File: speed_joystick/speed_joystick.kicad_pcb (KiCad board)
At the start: 2 copper layers, 89.2 x 61.1 mm, 67 parts, among them SW1 JS5208, U1 Teensy3.2, U2 SN65HVD230

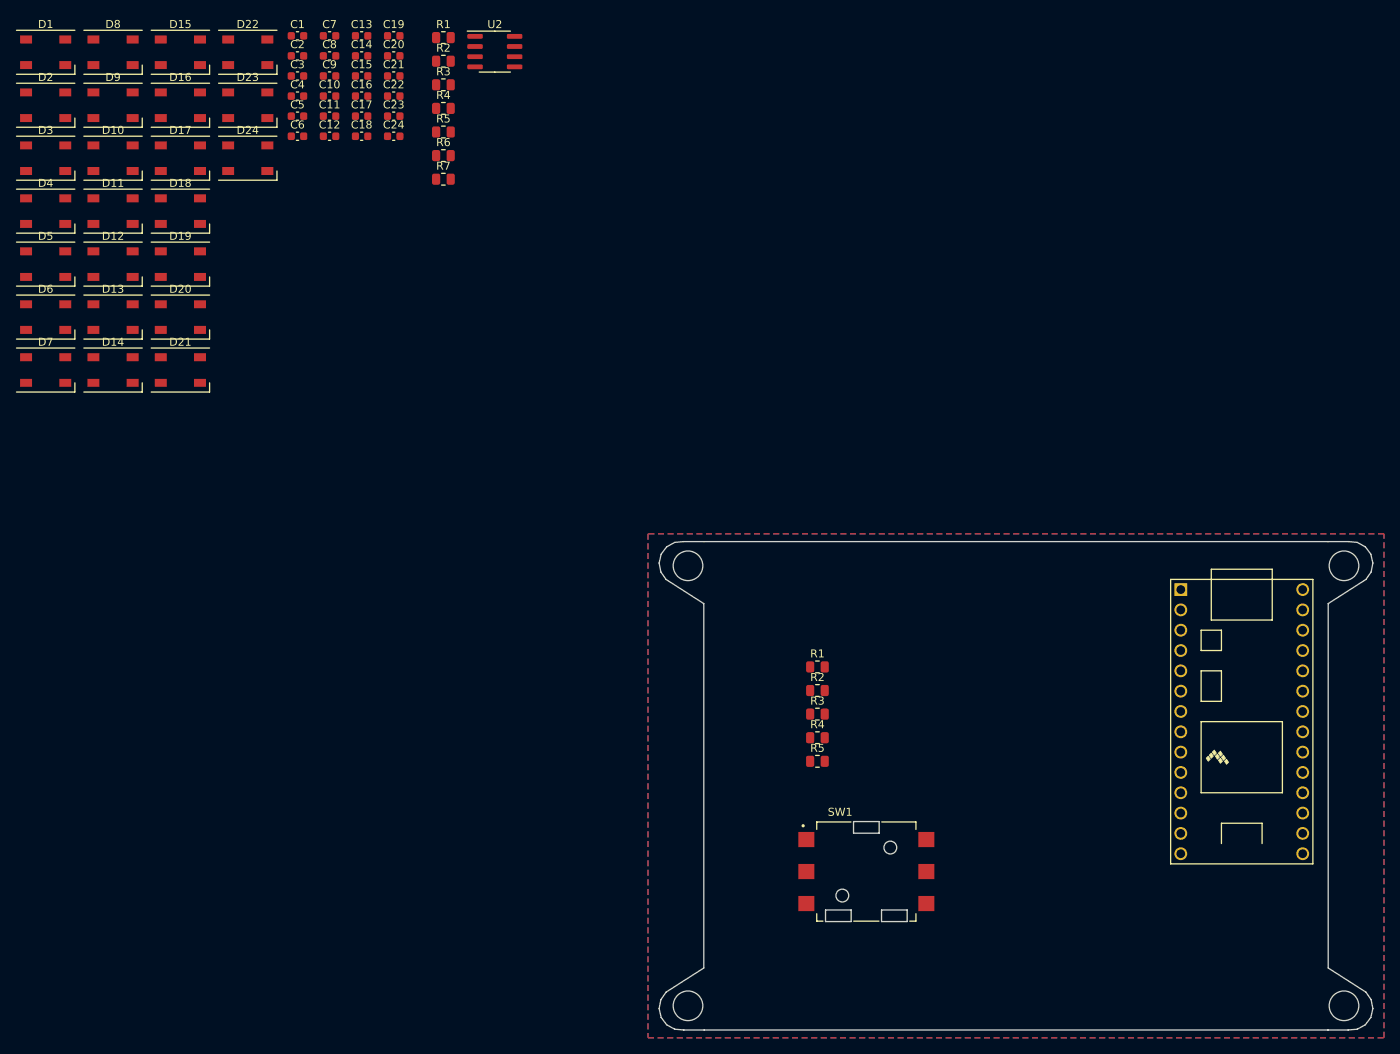
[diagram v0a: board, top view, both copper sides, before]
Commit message: work on speed_joystick pcb
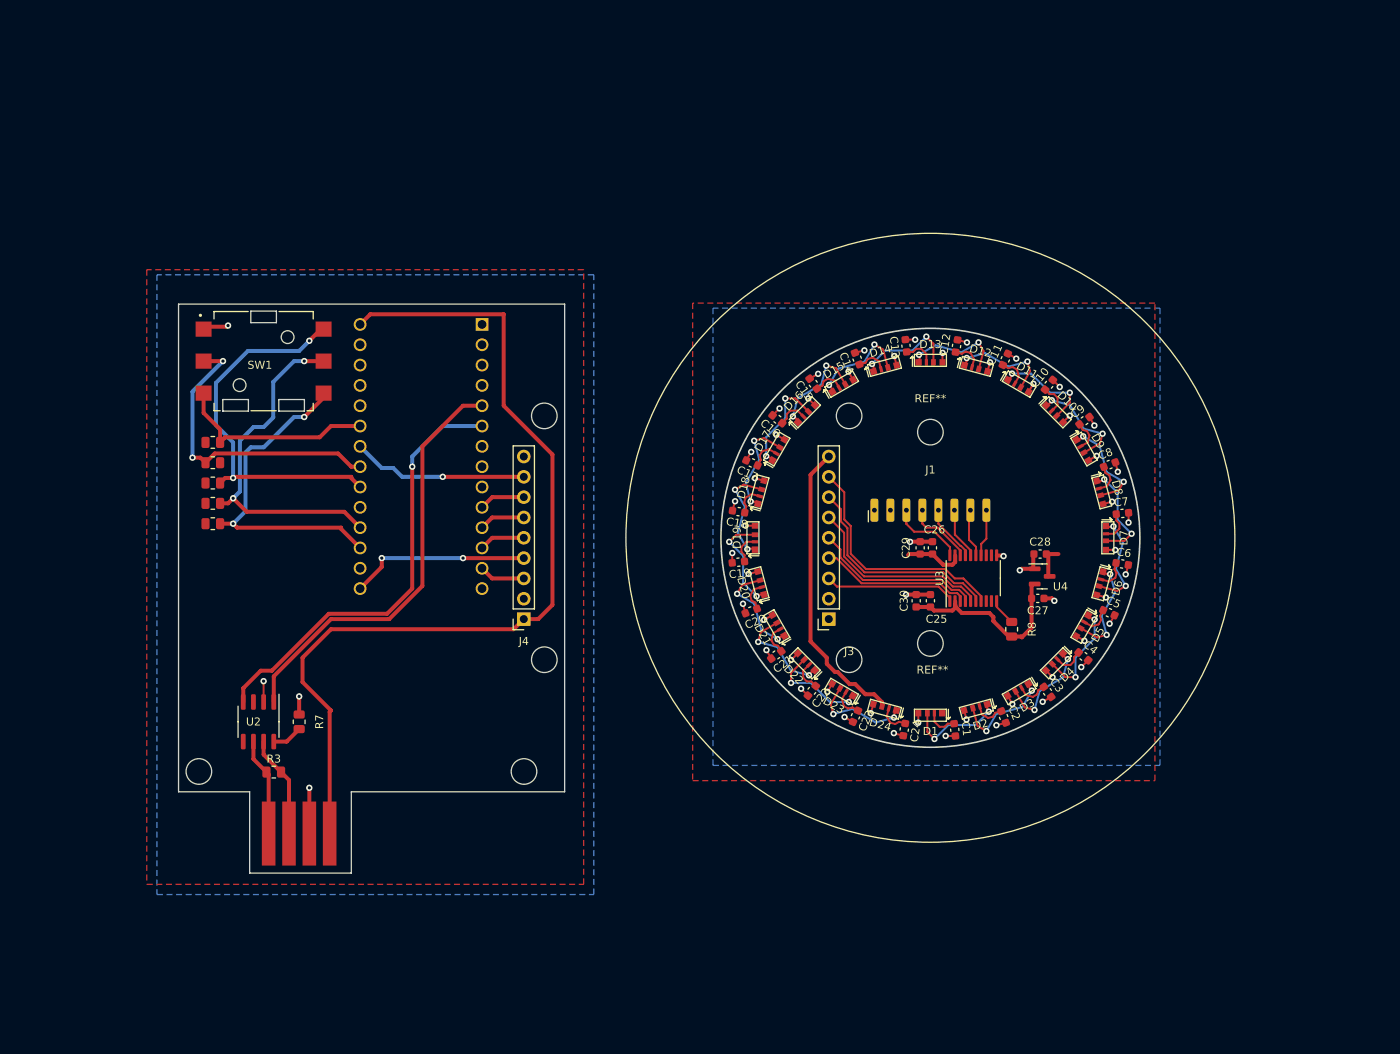
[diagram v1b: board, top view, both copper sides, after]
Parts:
- removed the R1 at (53.4, 0.97)
- removed the R1 at (100.2, 79.6)
- removed the R2 at (53.4, 3.92)
- removed the R2 at (100.2, 82.6)
- removed the R3 at (100.2, 85.5)
- removed the R3 at (53.4, 6.88)
- removed the R4 at (53.4, 9.82)
- removed the R4 at (100.2, 88.5)
- removed the R5 at (100.2, 91.4)
- removed the R5 at (53.4, 12.8)
- removed the REF** at (84.0, 67.0)
- removed the REF** at (84.0, 122.0)
- removed the REF** at (166.0, 122.0)
- removed the REF** at (166.0, 67.0)
- added ?: , , F.Cu at (66.0, 48.3)
- added ?: , , F.Cu at (63.5, 92.7)
- added ?: , , F.Cu at (104.1, 78.7)
- added ?: , , F.Cu at (66.0, 78.7)
- added ?: , , F.Cu at (104.1, 48.3)
- added ?: , , F.Cu at (22.9, 92.7)
- added C25: 0.1uF, Capacitor_SMD:C_0603_1608Metric, F.Cu at (114.3, 71.4)
- added C26: 0.1uF, Capacitor_SMD:C_0603_1608Metric, F.Cu at (114.6, 64.8)
- added C27: 1uF, Capacitor_SMD:C_0603_1608Metric, F.Cu at (127.7, 71.1)
- added C28: 1uF, Capacitor_SMD:C_0603_1608Metric, F.Cu at (128.0, 65.5)
- added C29: 10uF, Capacitor_SMD:C_0603_1608Metric, F.Cu at (113.0, 64.8)
- added C30: 10uF, Capacitor_SMD:C_0603_1608Metric, F.Cu at (112.5, 71.4)
- added J1: Conn_01x08, 8_hole:8_hole, F.Cu at (114.3, 60.0)
- added J2: Conn_01x04, 4pin:my_4_tab_edge, F.Cu at (31.6, 100.5)
- added J3: Conn_01x09, Connector_PinSocket_2.54mm:PinSocket_1x09_P2.54mm_Vertical, F.Cu at (101.6, 73.7)
- added J4: Conn_01x09, Connector_PinSocket_2.54mm:PinSocket_1x09_P2.54mm_Vertical, F.Cu at (63.5, 73.7)
- added R1: 10k, Resistor_SMD:R_0805_2012Metric, F.Cu at (24.6, 61.7)
- added R2: 10k, Resistor_SMD:R_0805_2012Metric, F.Cu at (24.6, 59.2)
- added R3: 120, Resistor_SMD:R_0805_2012Metric, F.Cu at (32.2, 92.8)
- added R4: 10k, Resistor_SMD:R_0805_2012Metric, F.Cu at (24.6, 56.7)
- added R5: 10k, Resistor_SMD:R_0805_2012Metric, F.Cu at (24.6, 51.6)
- added R8: R, Resistor_SMD:R_0805_2012Metric, F.Cu at (124.5, 74.9)
- added REF**: MountingHole_3.2mm_M3, MountingHole:MountingHole_3.2mm_M3, F.Cu at (114.3, 50.3)
- added REF**: MountingHole_3.2mm_M3, MountingHole:MountingHole_3.2mm_M3, F.Cu at (114.3, 76.7)
- added U3: 100k, Package_SO:TSSOP-20_4.4x6.5mm_P0.65mm, F.Cu at (119.7, 68.5)
- added U4: XC6206PxxxMR, Package_TO_SOT_SMD:SOT-23, F.Cu at (128.3, 68.3)
- D1, D10, D11, D12, D13, D14, D15, D16, D17, D18, D19, D2, D20, D21, D22, D23, D24, D3, D4, D5, D6, D7, D8, D9: footprint LED_SMD:LED_SK6812_PLCC4_5.0x5.0mm_P3.2mm -> LED_SMD:my_SK6812
- U1: moved to B.Cu
- moved D3 138.7 mm to (125.4, 82.7), turned to -150 degrees
- moved D2 138.7 mm to (120.0, 84.9), turned to -165 degrees
- moved D4 138.3 mm to (130.0, 79.2), turned to -135 degrees
- moved D1 138.2 mm to (114.3, 85.7), turned to 180 degrees
- moved D5 137.5 mm to (133.5, 74.6), turned to -120 degrees
- moved D6 136.2 mm to (135.7, 69.2), turned to -105 degrees
- moved D8 135.3 mm to (135.7, 57.8), turned to -75 degrees
- moved D7 134.4 mm to (136.5, 63.5), turned to -90 degrees
- moved D9 128.8 mm to (133.5, 52.4), turned to -60 degrees
- moved D10 122.1 mm to (130.0, 47.8), turned to -45 degrees
- moved C3 121.3 mm to (128.9, 82.8), turned to -54 degrees
- moved C2 120.9 mm to (123.5, 85.9), turned to -69 degrees
- moved C4 120.6 mm to (133.4, 78.3), turned to -39 degrees
- moved C1 119.5 mm to (117.3, 87.5), turned to -84 degrees
- moved C5 118.9 mm to (136.6, 72.9), turned to -24 degrees
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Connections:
- C1 pad 1: +3.3v -> R_+5V
- C1 pad 2: GND -> R_GND
- C10 pad 1: +3.3v -> R_+5V
- C10 pad 2: GND -> R_GND
- C11 pad 1: +3.3v -> R_+5V
- C11 pad 2: GND -> R_GND
- C12 pad 1: +3.3v -> R_+5V
- C12 pad 2: GND -> R_GND
- C13 pad 1: +3.3v -> R_+5V
- C13 pad 2: GND -> R_GND
- C14 pad 1: +3.3v -> R_+5V
- C14 pad 2: GND -> R_GND
- C15 pad 1: +3.3v -> R_+5V
- C15 pad 2: GND -> R_GND
- C16 pad 1: +3.3v -> R_+5V
- C16 pad 2: GND -> R_GND
- C17 pad 1: +3.3v -> R_+5V
- C17 pad 2: GND -> R_GND
- C18 pad 1: +3.3v -> R_+5V
- C18 pad 2: GND -> R_GND
- C19 pad 1: +3.3v -> R_+5V
- C19 pad 2: GND -> R_GND
- C2 pad 1: +3.3v -> R_+5V
- C2 pad 2: GND -> R_GND
- C20 pad 1: +3.3v -> R_+5V
- C20 pad 2: GND -> R_GND
- C21 pad 1: +3.3v -> R_+5V
- C21 pad 2: GND -> R_GND
- C22 pad 1: +3.3v -> R_+5V
- C22 pad 2: GND -> R_GND
- C23 pad 1: +3.3v -> R_+5V
- C23 pad 2: GND -> R_GND
- C24 pad 1: +3.3v -> R_+5V
- C24 pad 2: GND -> R_GND
- C3 pad 1: +3.3v -> R_+5V
- C3 pad 2: GND -> R_GND
- C4 pad 1: +3.3v -> R_+5V
- C4 pad 2: GND -> R_GND
- C5 pad 1: +3.3v -> R_+5V
- C5 pad 2: GND -> R_GND
- C6 pad 1: +3.3v -> R_+5V
- C6 pad 2: GND -> R_GND
- C7 pad 1: +3.3v -> R_+5V
- C7 pad 2: GND -> R_GND
- C8 pad 1: +3.3v -> R_+5V
- C8 pad 2: GND -> R_GND
- C9 pad 1: +3.3v -> R_+5V
- C9 pad 2: GND -> R_GND
- D1 pad 1: GND -> R_GND
- D1 pad 3: Net-(D1-VDD) -> R_+5V
- D1 pad 4: Net-(D1-DOUT) -> unconnected-(D1-DOUT-Pad4)
- D10 pad 1: GND -> R_GND
- D10 pad 3: unconnected-(D10-VDD-Pad3) -> R_+5V
- D11 pad 1: GND -> R_GND
- D11 pad 2: Net-(D10-DOUT) -> Net-(D11-DIN)
- D11 pad 3: +3.3v -> R_+5V
- D11 pad 4: Net-(D11-DOUT) -> Net-(D10-DIN)
- D12 pad 1: GND -> R_GND
- D12 pad 2: Net-(D11-DOUT) -> Net-(D12-DIN)
- D12 pad 3: +3.3v -> R_+5V
- D12 pad 4: Net-(D12-DOUT) -> Net-(D11-DIN)
- D13 pad 1: GND -> R_GND
- D13 pad 2: Net-(D12-DOUT) -> Net-(D13-DIN)
- D13 pad 3: +3.3v -> R_+5V
- D13 pad 4: Net-(D13-DOUT) -> Net-(D12-DIN)
- D14 pad 1: GND -> R_GND
- D14 pad 2: Net-(D13-DOUT) -> Net-(D14-DIN)
- D14 pad 3: +3.3v -> R_+5V
- D14 pad 4: unconnected-(D14-DOUT-Pad4) -> Net-(D13-DIN)
- D15 pad 1: GND -> R_GND
- D15 pad 2: unconnected-(D15-DIN-Pad2) -> Net-(D15-DIN)
- D15 pad 3: +3.3v -> R_+5V
- D15 pad 4: Net-(D15-DOUT) -> Net-(D14-DIN)
- D16 pad 1: GND -> R_GND
- D16 pad 2: Net-(D15-DOUT) -> Net-(D16-DIN)
- D16 pad 3: +3.3v -> R_+5V
- D16 pad 4: Net-(D1-DIN) -> Net-(D15-DIN)
- D17 pad 1: GND -> R_GND
- D17 pad 3: unconnected-(D17-VDD-Pad3) -> R_+5V
- D17 pad 4: Net-(D17-DOUT) -> Net-(D16-DIN)
- D18 pad 1: GND -> R_GND
- D18 pad 2: Net-(D17-DOUT) -> Net-(D18-DIN)
- D18 pad 3: unconnected-(D18-VDD-Pad3) -> R_+5V
- D18 pad 4: Net-(D18-DOUT) -> Net-(D17-DIN)
- D19 pad 1: GND -> R_GND
- D19 pad 2: Net-(D18-DOUT) -> Net-(D19-DIN)
- D19 pad 3: +3.3v -> R_+5V
- D19 pad 4: Net-(D19-DOUT) -> Net-(D18-DIN)
- D2 pad 1: GND -> R_GND
- D2 pad 2: Net-(D1-DOUT) -> Net-(D2-DIN)
- D2 pad 3: Net-(D1-VDD) -> R_+5V
- D2 pad 4: Net-(D2-DOUT) -> Net-(D1-DIN)
- D20 pad 1: GND -> R_GND
- D20 pad 2: Net-(D19-DOUT) -> Net-(D20-DIN)
- D20 pad 3: +3.3v -> R_+5V
- D20 pad 4: Net-(D20-DOUT) -> Net-(D19-DIN)
- D21 pad 1: GND -> R_GND
- D21 pad 2: Net-(D20-DOUT) -> Net-(D21-DIN)
- D21 pad 3: +3.3v -> R_+5V
- D21 pad 4: Net-(D21-DOUT) -> Net-(D20-DIN)
- D22 pad 1: GND -> R_GND
- D22 pad 2: Net-(D21-DOUT) -> Net-(D22-DIN)
- D22 pad 3: +3.3v -> R_+5V
- D22 pad 4: unconnected-(D22-DOUT-Pad4) -> Net-(D21-DIN)
- D23 pad 1: GND -> R_GND
- D23 pad 2: unconnected-(D23-DIN-Pad2) -> Net-(D23-DIN)
- D23 pad 3: +3.3v -> R_+5V
- D23 pad 4: Net-(D23-DOUT) -> Net-(D22-DIN)
- D24 pad 1: GND -> R_GND
- D24 pad 2: Net-(D23-DOUT) -> R_DIN
- D24 pad 3: +3.3v -> R_+5V
- D24 pad 4: unconnected-(D24-DOUT-Pad4) -> Net-(D23-DIN)
- D3 pad 1: GND -> R_GND
- D3 pad 2: Net-(D2-DOUT) -> Net-(D3-DIN)
- D3 pad 3: Net-(D1-VDD) -> R_+5V
- D3 pad 4: Net-(D3-DOUT) -> Net-(D2-DIN)
- D4 pad 1: GND -> R_GND
- D4 pad 2: Net-(D3-DOUT) -> Net-(D4-DIN)
- D4 pad 3: unconnected-(D4-VDD-Pad3) -> R_+5V
- D4 pad 4: Net-(D17-DIN) -> Net-(D3-DIN)
- D5 pad 1: GND -> R_GND
- D5 pad 2: unconnected-(D5-DIN-Pad2) -> Net-(D5-DIN)
- D5 pad 3: Net-(D5-VDD) -> R_+5V
- D5 pad 4: Net-(D5-DOUT) -> Net-(D4-DIN)
- D6 pad 1: GND -> R_GND
- D6 pad 2: Net-(D5-DOUT) -> Net-(D6-DIN)
- D6 pad 3: Net-(D5-VDD) -> R_+5V
- D6 pad 4: Net-(D6-DOUT) -> Net-(D5-DIN)
- D7 pad 1: GND -> R_GND
- D7 pad 2: Net-(D6-DOUT) -> Net-(D7-DIN)
- D7 pad 3: Net-(D5-VDD) -> R_+5V
- D7 pad 4: Net-(D7-DOUT) -> Net-(D6-DIN)
- D8 pad 1: GND -> R_GND
- D8 pad 2: Net-(D7-DOUT) -> Net-(D8-DIN)
- D8 pad 3: unconnected-(D8-VDD-Pad3) -> R_+5V
- D8 pad 4: Net-(D8-DOUT) -> Net-(D7-DIN)
- D9 pad 1: GND -> R_GND
- D9 pad 2: Net-(D8-DOUT) -> Net-(D10-DOUT)
- D9 pad 3: unconnected-(D9-VDD-Pad3) -> R_+5V
- D9 pad 4: Net-(D10-DIN) -> Net-(D8-DIN)
- R6 pad 1: +3.3v -> +3.3V
- U1 pad 10: RST -> RES
- U1 pad 11: RS/DC -> DC
- U1 pad 21: P_IN -> unconnected-(U1-14_A0_SCK-Pad21)
- U1 pad 22: unconnected-(U1-15_A1_CS_Touch-Pad22) -> B5
- U1 pad 23: unconnected-(U1-16_A2_SCL0_Touch-Pad23) -> B4
- U1 pad 24: unconnected-(U1-17_A3_SDA0_Touch-Pad24) -> DIN_SIG
- U1 pad 25: unconnected-(U1-18_A4_SDA0_Touch-Pad25) -> B3
- U1 pad 26: unconnected-(U1-19_A5_SCL0_Touch-Pad26) -> B1
- U1 pad 27: unconnected-(U1-20_A6_CS_PWM-Pad27) -> BL
- U1 pad 28: unconnected-(U1-21_A7_RX1_CS_PWM-Pad28) -> B2
- U1 pad 31: +3.3v -> +3.3V
- U1 pad 33: unconnected-(U1-Vin-Pad33) -> +5V
- U1 pad 4: B1 -> unconnected-(U1-2-Pad4)
- U1 pad 7: B4 -> unconnected-(U1-5_TX1_PWM-Pad7)
- U1 pad 8: B3 -> unconnected-(U1-6_PWM-Pad8)
- U2 pad 3: +3.3v -> +3.3V
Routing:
- net +5V: track 0.00 -> 114.8 mm
- net R_+5V: track 0.00 -> 106.6 mm
- net R_GND: track 0.00 -> 69.1 mm, vias 0 -> 53
- net CAN_RX: track 0.00 -> 54.8 mm, vias 0 -> 1
- net CAN_TX: track 0.00 -> 53.5 mm
- net B3: track 0.00 -> 47.5 mm, vias 0 -> 2
- net B4: track 0.00 -> 44.0 mm, vias 0 -> 2
- net B5: track 0.00 -> 41.6 mm, vias 0 -> 2
- net B1: track 0.00 -> 38.4 mm, vias 0 -> 2
- net R_DIN: track 0.00 -> 37.1 mm
- net R_BL: track 0.00 -> 29.9 mm
- net R_RES: track 0.00 -> 27.1 mm
- net B2: track 0.00 -> 25.4 mm
- net R_DC: track 0.00 -> 24.2 mm
- net R_+3.3V: track 0.00 -> 23.7 mm
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- added copper zone on F.Cu, net +3.3V
- added copper zone on F.Cu, net R_+5V
- added copper zone on B.Cu, net R_GND
- removed copper zone on F.Cu, net +3.3v
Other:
- board size 89.2 x 61.1 mm -> 120.2 x 71.1 mm
- board text added: "SPEED JOYSTICK V1.0"
